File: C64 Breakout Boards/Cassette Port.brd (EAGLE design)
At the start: 35.6 x 25.4 mm, 1 part

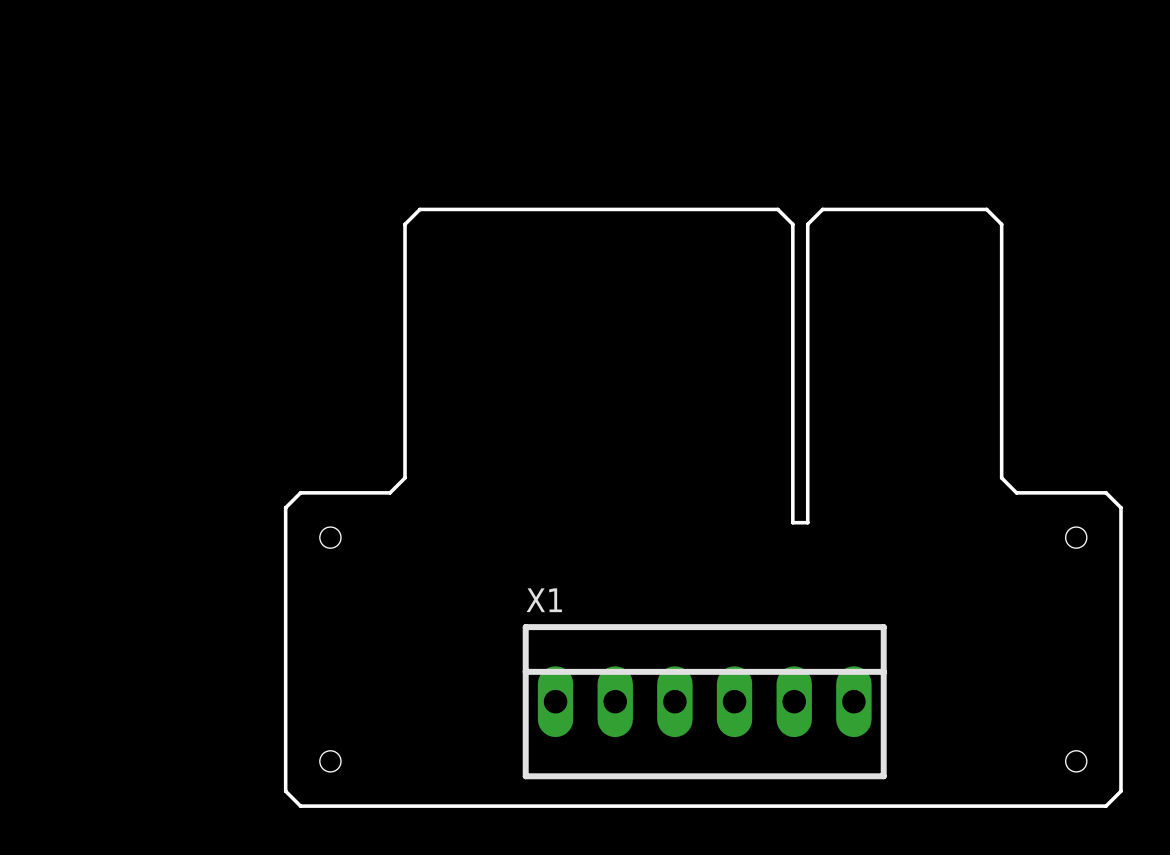
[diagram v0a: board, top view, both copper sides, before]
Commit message: Breakout Boards done
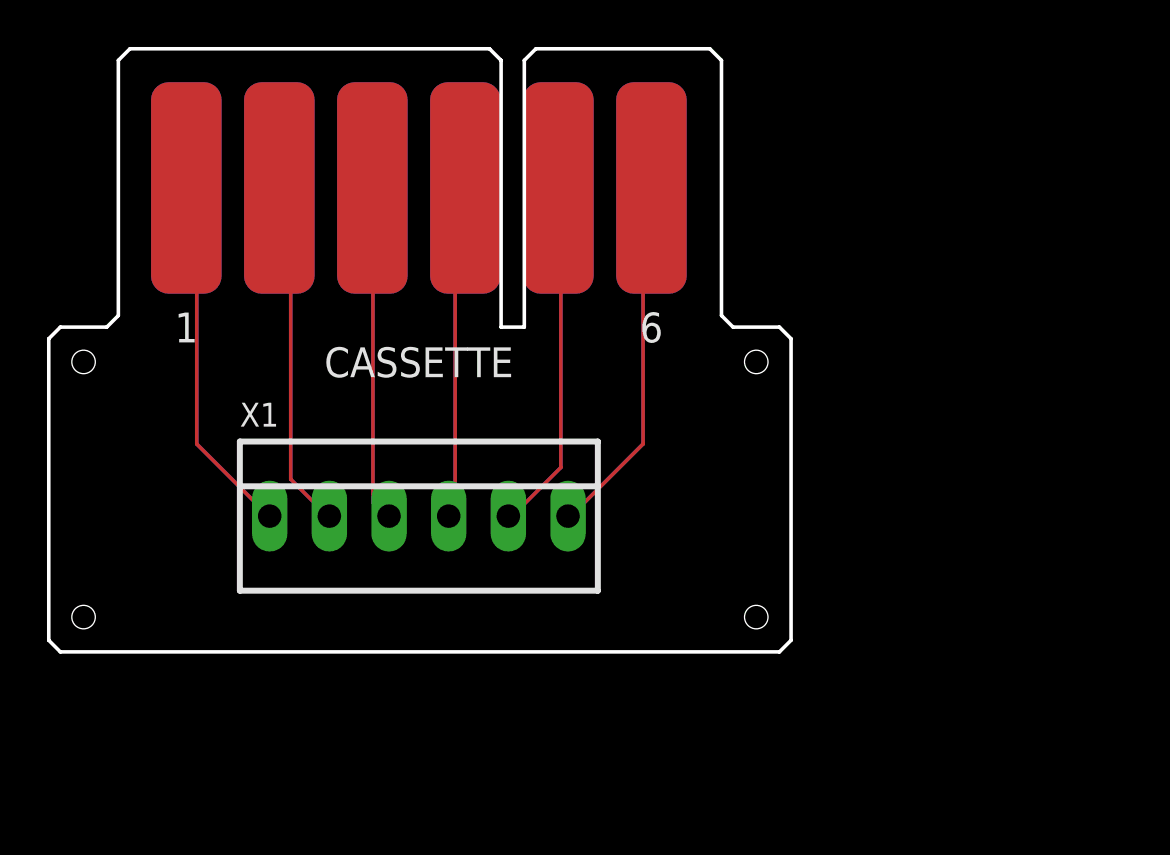
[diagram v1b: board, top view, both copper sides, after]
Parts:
- added CASSETTE: C64_CASSETTE, myparts:C64_CASSETTE
- moved X1 14.5 mm to (-0.04, -6.07)
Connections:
- removed net GND1: X1.1
- removed net MOTOR1: X1.3
- removed net READ1: X1.4
- removed net SENSE1: X1.6
- removed net VCC1: X1.2
- removed net WRITE1: X1.5
- new net N$1: CASSETTE.GND1, CASSETTE.GND2, X1.1
- new net N$11: CASSETTE.SENSE1, CASSETTE.SENSE2, X1.6
- new net N$3: CASSETTE.VCC1, CASSETTE.VCC2, X1.2
- new net N$5: CASSETTE.MOTOR1, CASSETTE.MOTOR2, X1.3
- new net N$7: CASSETTE.READ1, CASSETTE.READ2, X1.4
- new net N$9: CASSETTE.WRITE1, CASSETTE.WRITE2, X1.5
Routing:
- net N$11: track 0.00 -> 31.0 mm
- net N$1: track 0.00 -> 30.9 mm
- net N$9: track 0.00 -> 30.0 mm
- net N$3: track 0.00 -> 29.8 mm
- net N$7: track 0.00 -> 28.7 mm
- net N$5: track 0.00 -> 28.6 mm
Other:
- board size 35.6 x 25.4 mm -> 31.6 x 25.7 mm
